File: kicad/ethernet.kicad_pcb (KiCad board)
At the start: 2 copper layers, 6 parts, among them J1 RJ45_Abracon_ARJP11A-MASA-B-A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, U1 TM4C1294NCPDTI3

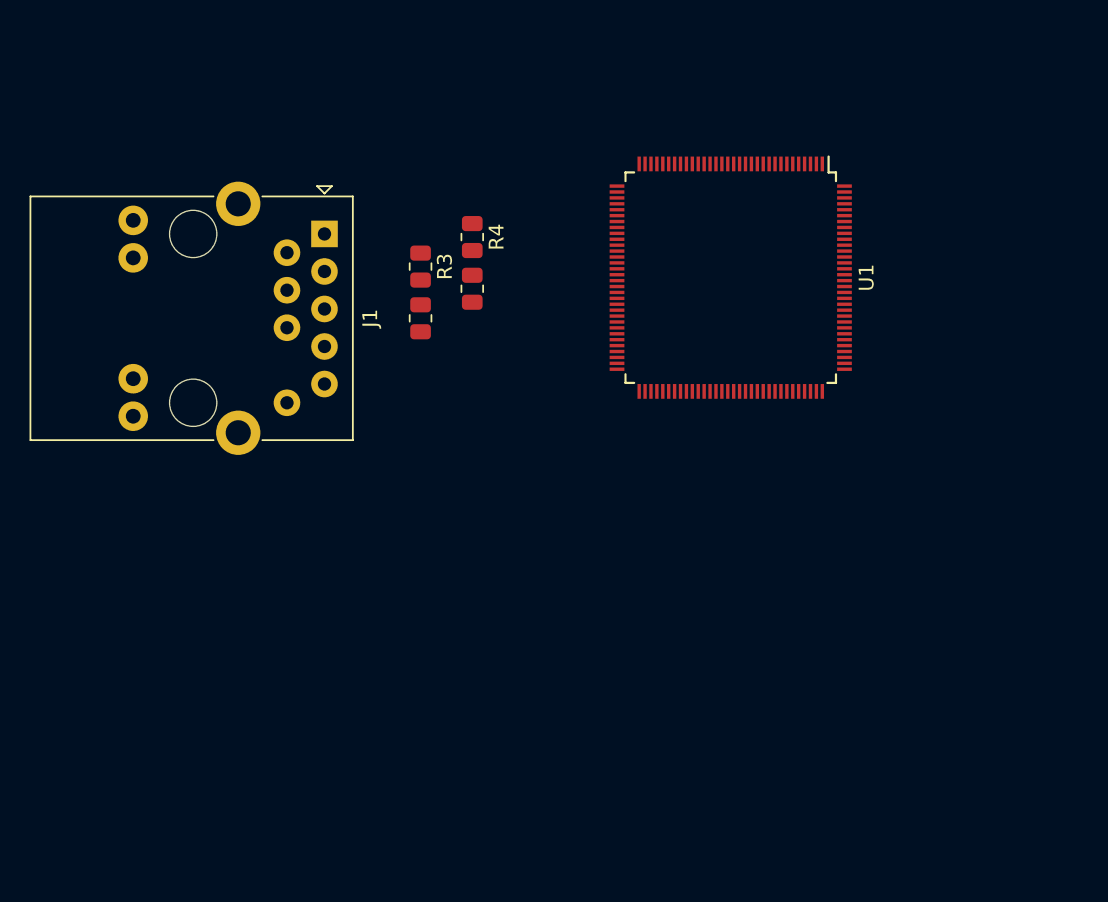
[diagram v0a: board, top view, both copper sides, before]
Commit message: board layout
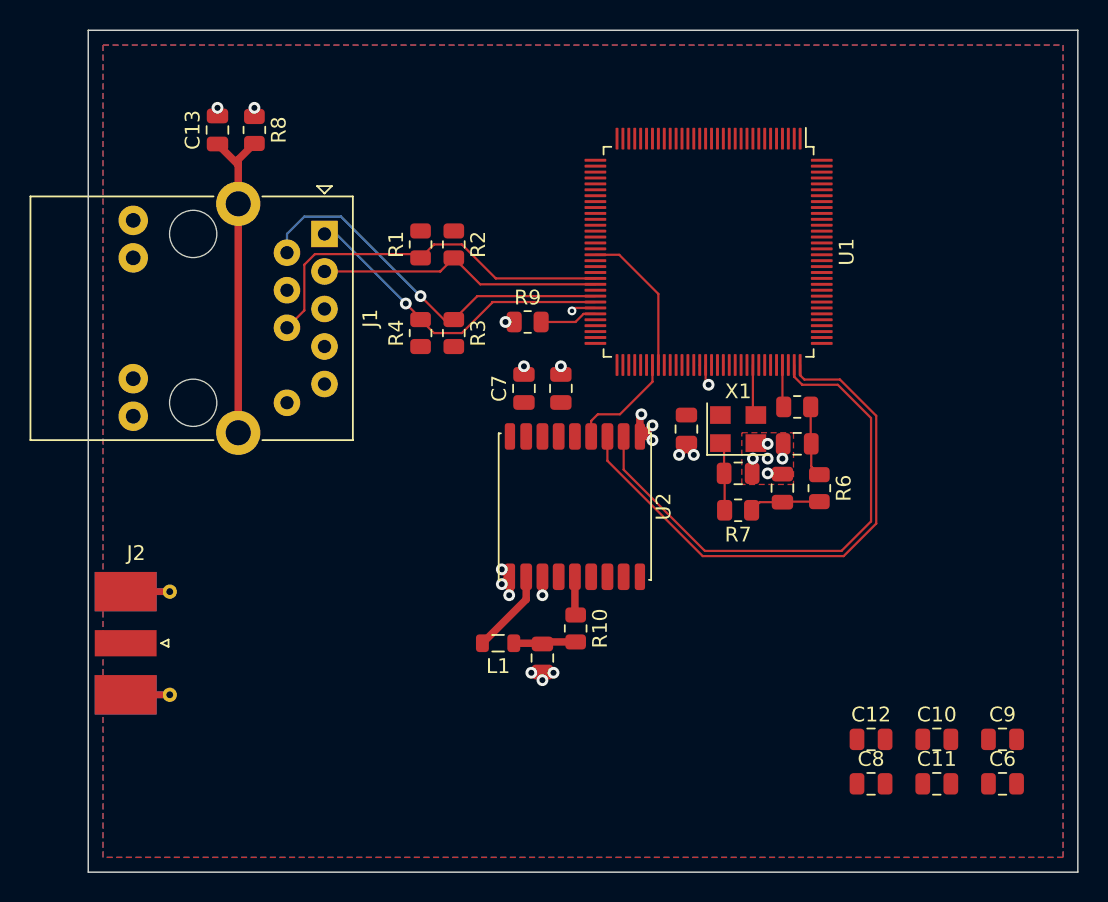
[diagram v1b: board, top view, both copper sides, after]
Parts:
- added C1: 100n, Capacitor_SMD:C_0805_2012Metric, F.Cu at (71.0, 41.0)
- added C10: 100n, Capacitor_SMD:C_0805_2012Metric, F.Cu at (80.5, 61.0)
- added C11: 100n, Capacitor_SMD:C_0805_2012Metric, F.Cu at (80.5, 64.0)
- added C12: 100n, Capacitor_SMD:C_0805_2012Metric, F.Cu at (76.0, 61.0)
- added C13: 4.7n, Capacitor_SMD:C_0805_2012Metric, F.Cu at (31.8, 19.8)
- added C14: 10n, Capacitor_SMD:C_0805_2012Metric, F.Cu at (53.8, 55.5)
- added C2: 100n, Capacitor_SMD:C_0805_2012Metric, F.Cu at (70.0, 44.0)
- added C3: 100n, Capacitor_SMD:C_0805_2012Metric, F.Cu at (67.0, 43.0)
- added C4: 100n, Capacitor_SMD:C_0805_2012Metric, F.Cu at (63.5, 40.0)
- added C5: 100n, Capacitor_SMD:C_0805_2012Metric, F.Cu at (55.0, 37.2)
- added C6: 100n, Capacitor_SMD:C_0805_2012Metric, F.Cu at (84.9, 64.0)
- added C7: 100n, Capacitor_SMD:C_0805_2012Metric, F.Cu at (52.5, 37.2)
- added C8: 100n, Capacitor_SMD:C_0805_2012Metric, F.Cu at (76.0, 64.0)
- added C9: 100n, Capacitor_SMD:C_0805_2012Metric, F.Cu at (84.9, 61.0)
- added J2: Conn_Coaxial, Connector_Coaxial:SMA_Molex_73251-2120_EdgeMount_Horizontal, F.Cu at (25.5, 54.5)
- added L1: 27n, Inductor_SMD:L_0805_2012Metric, F.Cu at (50.8, 54.5)
- added R10: 10, Resistor_SMD:R_0805_2012Metric, F.Cu at (56.0, 53.5)
- added R5: 10k, Resistor_SMD:R_0805_2012Metric, F.Cu at (71.0, 38.5)
- added R6: 10k, Resistor_SMD:R_0805_2012Metric, F.Cu at (72.5, 44.0)
- added R7: 10k, Resistor_SMD:R_0805_2012Metric, F.Cu at (67.0, 45.5)
- added R8: 1M, Resistor_SMD:R_0805_2012Metric, F.Cu at (34.2, 19.8)
- added R9: 4.87k, Resistor_SMD:R_0805_2012Metric, F.Cu at (52.8, 32.8)
- added U2: MAX-8Q, RF_GPS:ublox_MAX, F.Cu at (56.0, 45.2)
- added X1: TXEAADSANF-25.000000, Oscillator:Oscillator_SMD_SeikoEpson_SG8002CE-4Pin_3.2x2.5mm, F.Cu at (67.0, 40.0)
- U1: value TM4C1294NCPDTI3 -> MSP432E401Y; footprint Package_QFP:TQFP-128_14x14mm_P0.4mm -> Package_QFP:LQFP-128_14x14mm_P0.4mm
- moved R4 7.38 mm to (45.5, 33.5), turned to 90 degrees
- moved R3 5.03 mm to (47.8, 33.5)
- moved R1 5.00 mm to (45.5, 27.5)
- moved R2 3.25 mm to (47.8, 27.5), turned to -90 degrees
- moved U1 2.30 mm to (65.0, 28.0)
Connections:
- J1 pad 15: unconnected-(J1-Pad15) -> Net-(J1-Pad15)
- U1 pad 101: unconnected-(U1-Pad101) -> +3V3
- U1 pad 113: unconnected-(U1-Pad113) -> +3V3
- U1 pad 122: unconnected-(U1-Pad122) -> +3V3
- U1 pad 16: unconnected-(U1-Pad16) -> +3V3
- U1 pad 26: unconnected-(U1-Pad26) -> +3V3
- U1 pad 28: unconnected-(U1-Pad28) -> +3V3
- U1 pad 39: unconnected-(U1-Pad39) -> +3V3
- U1 pad 47: unconnected-(U1-Pad47) -> +3V3
- U1 pad 49: unconnected-(U1-Pad49) -> uPPS
- U1 pad 51: unconnected-(U1-Pad51) -> +3V3
- U1 pad 52: unconnected-(U1-Pad52) -> +3V3
- U1 pad 59: unconnected-(U1-Pad59) -> Net-(U1-Pad59)
- U1 pad 69: unconnected-(U1-Pad69) -> +3V3
- U1 pad 7: unconnected-(U1-Pad7) -> +3V3
- U1 pad 71: unconnected-(U1-Pad71) -> gPPS
- U1 pad 72: unconnected-(U1-Pad72) -> uPPS
- U1 pad 79: unconnected-(U1-Pad79) -> +3V3
- U1 pad 88: unconnected-(U1-Pad88) -> Net-(U1-Pad88)
- U1 pad 90: unconnected-(U1-Pad90) -> +3V3
- U1 pad 93: unconnected-(U1-Pad93) -> Net-(U1-Pad93)
- U1 pad 95: unconnected-(U1-Pad95) -> gTX
- U1 pad 96: unconnected-(U1-Pad96) -> gRX
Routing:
- net gRX: track 0.00 -> 37.7 mm
- net gTX: track 0.00 -> 36.3 mm
- net Net-(J1-Pad6): track 0.00 -> 26.2 mm
- net Net-(J1-Pad2): track 0.00 -> 26.2 mm, vias 0 -> 1
- net Net-(J1-Pad1): track 0.00 -> 22.1 mm, vias 0 -> 1
- net Net-(J1-Pad15): track 0.00 -> 22.0 mm
- net Net-(J1-Pad3): track 0.00 -> 19.5 mm
- net GND: track 0.00 -> 12.4 mm, vias 0 -> 24
- net uPPS: track 0.00 -> 10.2 mm
- net gPPS: track 0.00 -> 7.44 mm
- net Net-(U2-Pad11): track 0.00 -> 5.73 mm
- net Net-(C2-Pad1): track 0.00 -> 4.83 mm
- net Net-(C1-Pad1): track 0.00 -> 4.83 mm
- net Net-(C3-Pad1): track 0.00 -> 4.67 mm
- net Net-(C14-Pad1): track 0.00 -> 4.27 mm
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- added copper zone on F.Cu, net +3V3
- added copper zone on B.Cu, net GND
- added copper zone on F.Cu, net GND
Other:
- board outline added: 67 x 57 mm
